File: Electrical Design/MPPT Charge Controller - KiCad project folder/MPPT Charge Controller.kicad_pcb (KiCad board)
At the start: 4 copper layers, 32 x 80 mm, 75 parts, among them J1 Conn_01x02_Socket, J2 Conn_01x02_Socket, J3 Conn_01x02_Socket, Q1 Q_Dual_NMOS_S1G1S2G2D2D2D1D1, Q2 Q_Dual_NMOS_S1G1S2G2D2D2D1D1, Q3 2N7002, U2 AP63203WU, U3 ACS712, U4 ACS712, U5 MCP4018

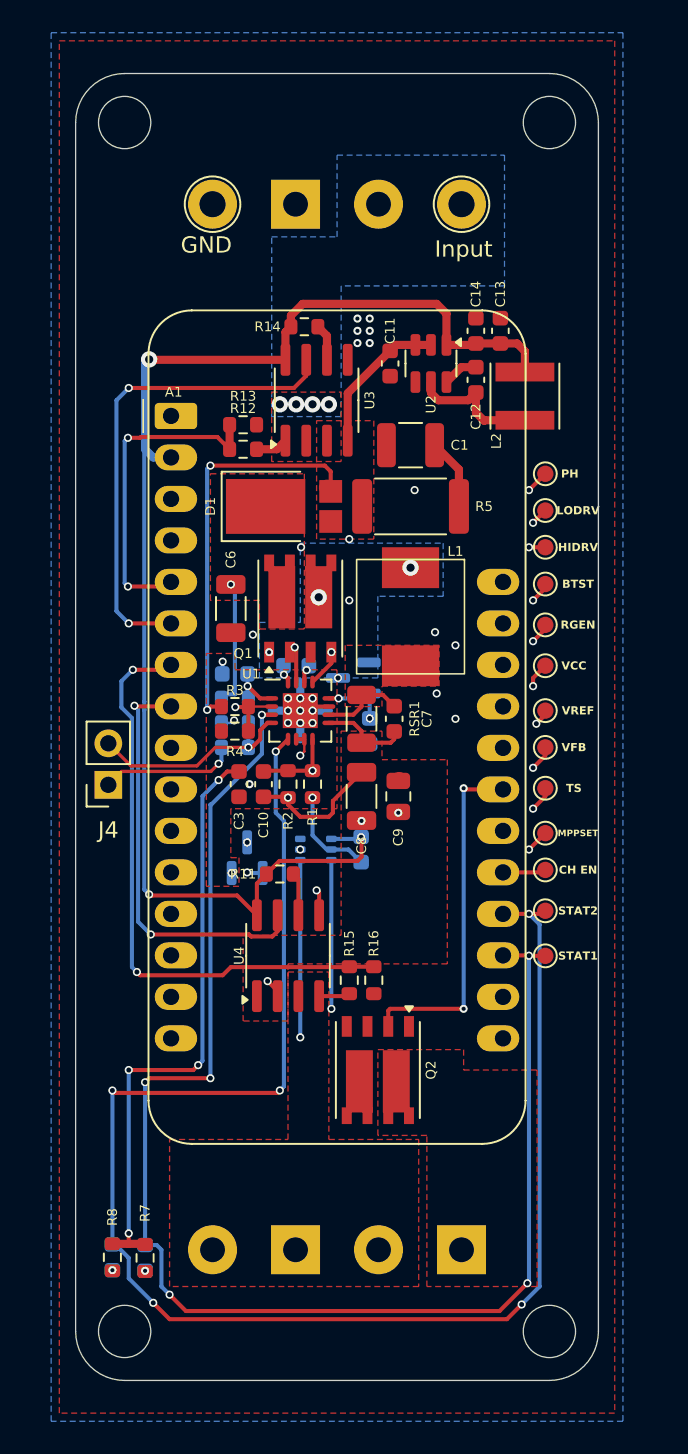
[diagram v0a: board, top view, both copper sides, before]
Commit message: continue to adapt for MEGAphone
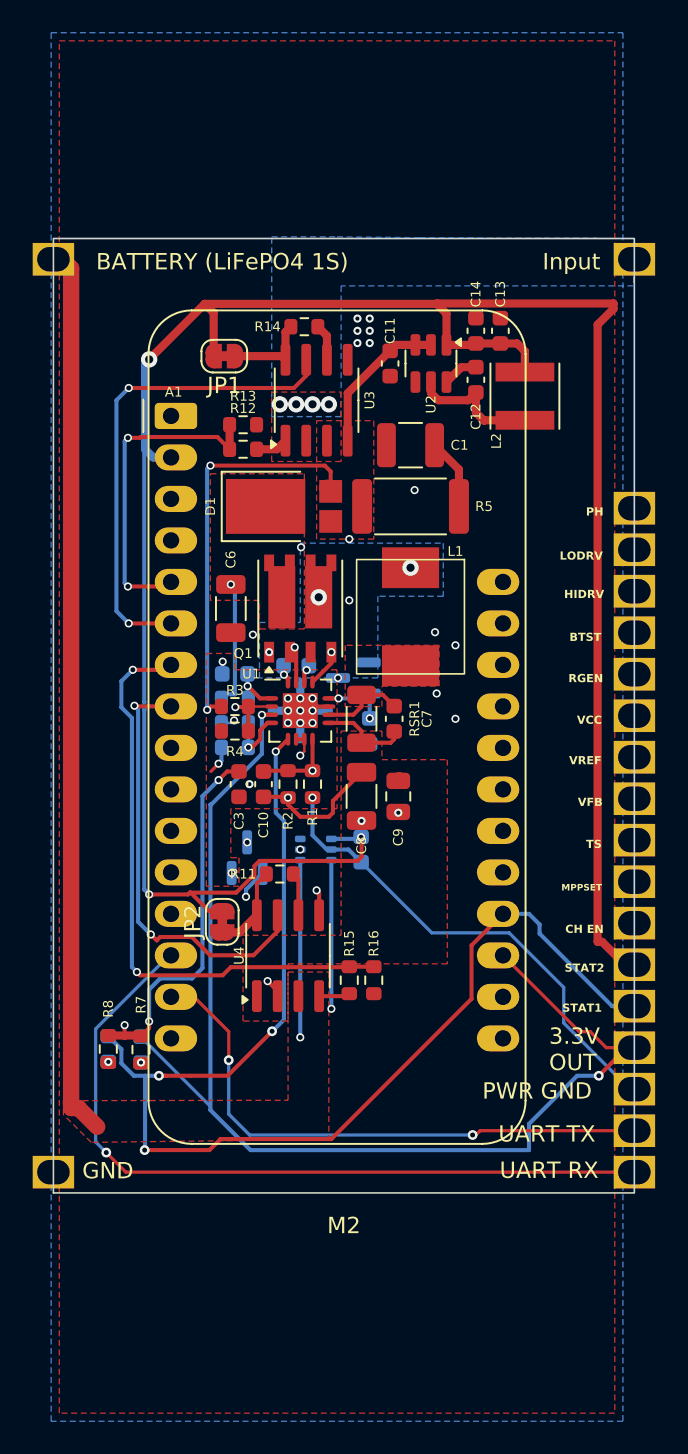
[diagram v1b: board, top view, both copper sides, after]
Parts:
- removed ? (x3): , 
- removed G***: LOGO, New Logo:byteSizedEngineeringLogo-5mm
- removed J1, J2, J3: Conn_01x02_Socket, TerminalBlock:TerminalBlock_bornier-2_P5.08mm
- removed J4: ~, Connector_PinSocket_2.54mm:PinSocket_1x02_P2.54mm_Vertical
- removed Q2: Q_Dual_NMOS_S1G1S2G2D2D2D1D1, Package_SO:PowerPAK_SO-8_Dual
- removed REF**: MountingHole_3.2mm_M3, MountingHole:MountingHole_3.2mm_M3
- removed TP1, TP10, TP11, TP12, TP13, TP2, TP3, TP4, TP5, TP6, TP7, TP8, TP9: TestPoint, TestPoint:TestPoint_Pad_D1.0mm
- removed TP14, TP15: TestPoint, TestPoint:TestPoint_Loop_D2.60mm_Drill1.6mm_Beaded
- added JP1: Jumper_2_Bridged, Jumper:SolderJumper-2_P1.3mm_Bridged_RoundedPad1.0x1.5mm, F.Cu at (103.1, 77.3)
- added JP2: Jumper_2_Bridged, Jumper:SolderJumper-2_P1.3mm_Bridged_RoundedPad1.0x1.5mm, F.Cu at (103.0, 111.9)
- added M2: ~, MegaCastle:MegaCastle2x23-Module-I30.0x53.6-M80000307FFFC, F.Cu at (110.4, 99.3)
- RSR1: value 0.02 -> 0.01
- moved D3 12.8 mm to (98.0, 119.8)
- moved D4 12.8 mm to (96.0, 119.7)
- moved R7 12.8 mm to (98.0, 119.8)
- moved R8 12.8 mm to (96.0, 119.7)
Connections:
- net Net-(J2-Pin_2) renamed VBAT_OUT
- net PWR GND renamed PWR_GND
- A1 pad 14: unconnected-(A1-RX/IO16-Pad14) -> UART_RX
- A1 pad 15: unconnected-(A1-TX/IO17-Pad15) -> UART_TX
- A1 pad 23: /Load Enable -> unconnected-(A1-D11-Pad23)
- R11 pad 2: +3.3V -> VCC_ACS712_2
- R14 pad 2: +3.3V -> VCC_ACS712
- U3 pad 8: +3.3V -> VCC_ACS712
- U4 pad 8: +3.3V -> VCC_ACS712_2
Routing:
- net +3.3V: track 83.5 -> 139.6 mm
- net VBAT_OUT: track 1.91 -> 56.7 mm
- net UART_RX: track 0.00 -> 47.1 mm, vias 0 -> 1
- net UART_TX: track 0.00 -> 34.9 mm, vias 0 -> 2
- net /Load Enable: track 21.6 -> 0.00 mm, vias 2 -> 0
- net /STAT2: track 97.3 -> 77.3 mm, vias 6 -> 4
- net PWR_GND: track 16.2 -> 33.3 mm
- net /STAT1: track 88.0 -> 73.6 mm, vias 6 -> 2
- net /~{Charge EN}: track 19.3 -> 27.6 mm
- net /VREF: track 55.3 -> 47.4 mm, vias 7 -> 5
- net /HIDRV: track 23.6 -> 30.0 mm, vias 3 -> 2
- net /MPPSET: track 31.6 -> 37.4 mm, vias 4 -> 3
- net /LODRV: track 22.4 -> 28.2 mm, vias 3 -> 2
- net /BTST: track 22.2 -> 28.0 mm, vias 4 -> 3
- net /RGEN: track 20.0 -> 25.6 mm, vias 5 -> 4
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- removed copper zone on F.Cu, net Net-(J3-Pin_1)
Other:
- board size 32 x 80 mm -> 35.6 x 58.4 mm
- board text added: "3.3V OUT"
- board text added: "BATTERY (LiFePO4 1S)"
- board text added: "PWR GND"
- board text added: "UART RX"
- board text added: "UART TX"
- board text removed: "- + 12V Battery"
- board text removed: "- + 12V Load"
- board text removed: "- + 5V-28V Solar Input"
